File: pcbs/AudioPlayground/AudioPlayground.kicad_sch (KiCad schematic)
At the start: 0 parts

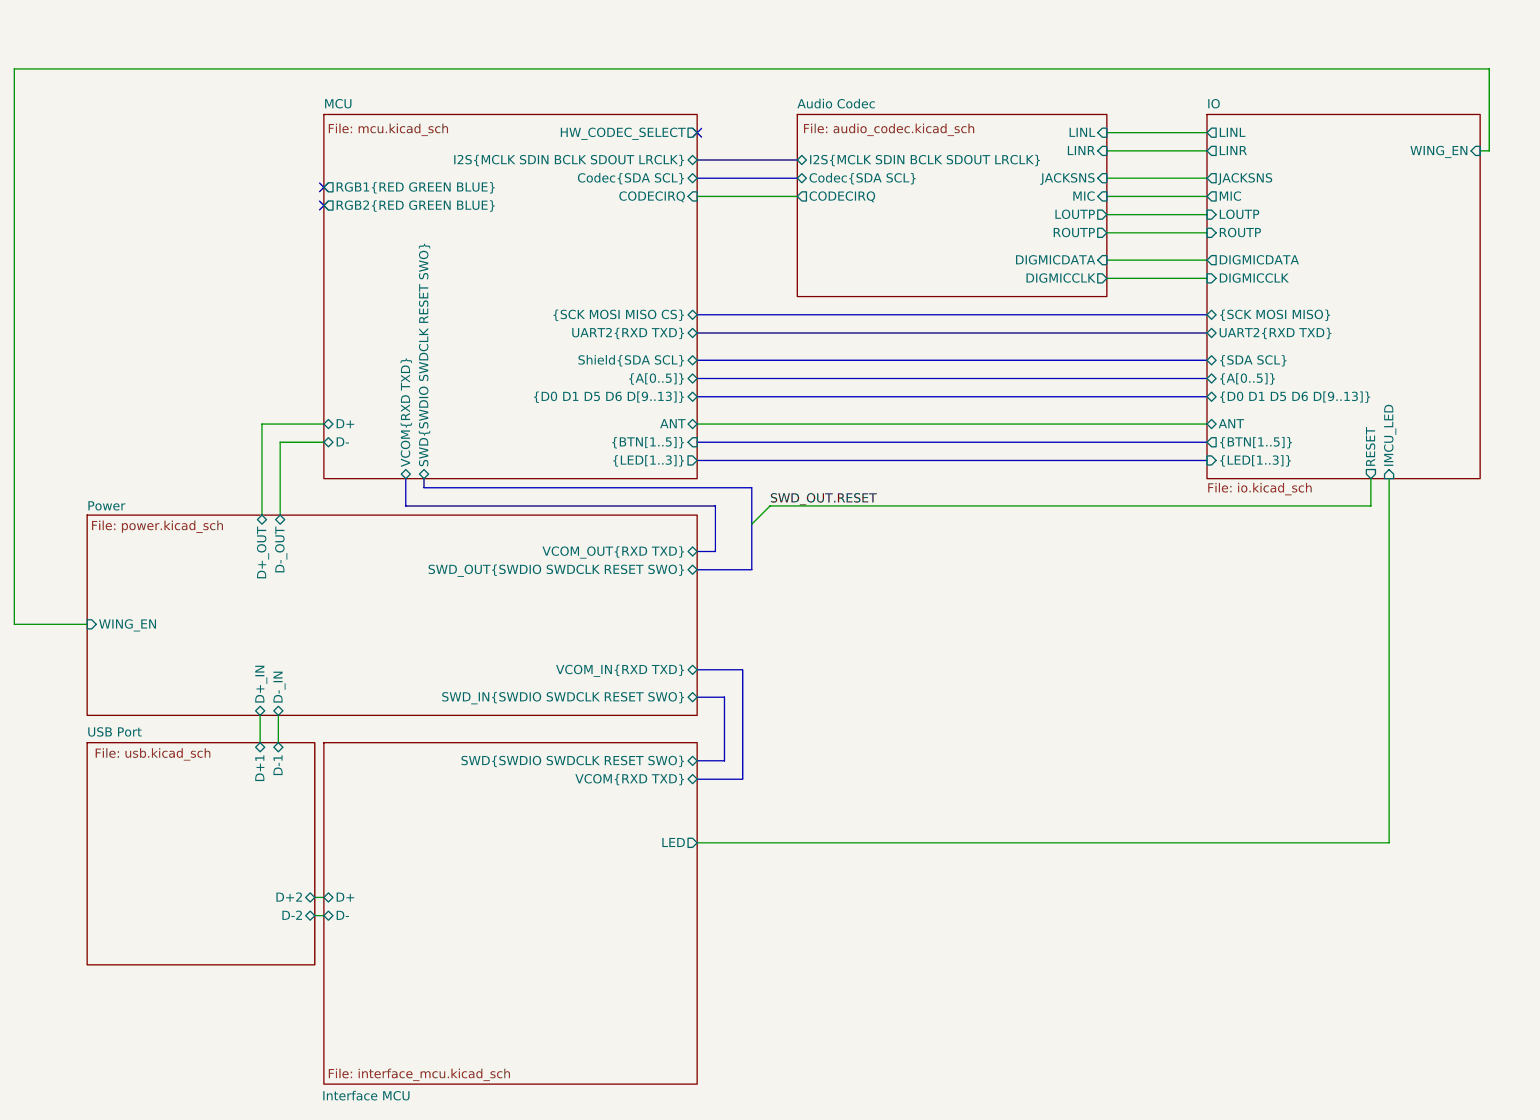
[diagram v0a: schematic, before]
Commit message: Improve Optic
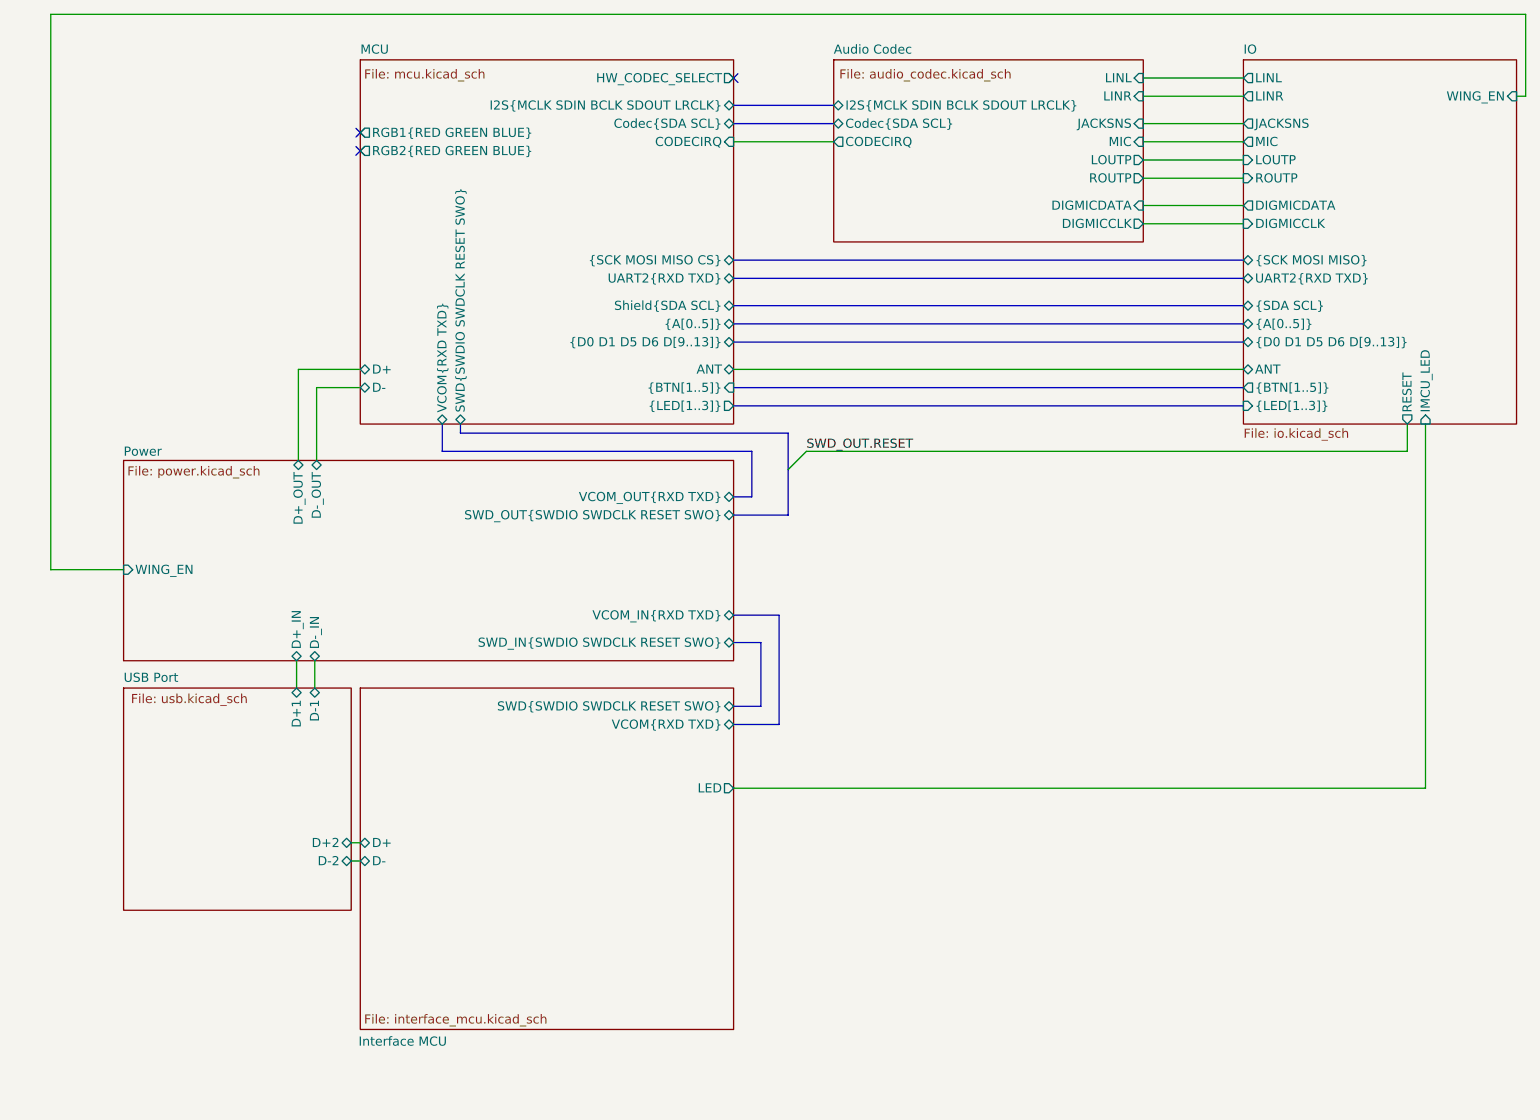
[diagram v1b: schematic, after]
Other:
- title: BLE Audio Devboard -> LE Audio Playground
